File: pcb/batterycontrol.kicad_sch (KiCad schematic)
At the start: 4 parts, among them SW1 MST22D18G2_125

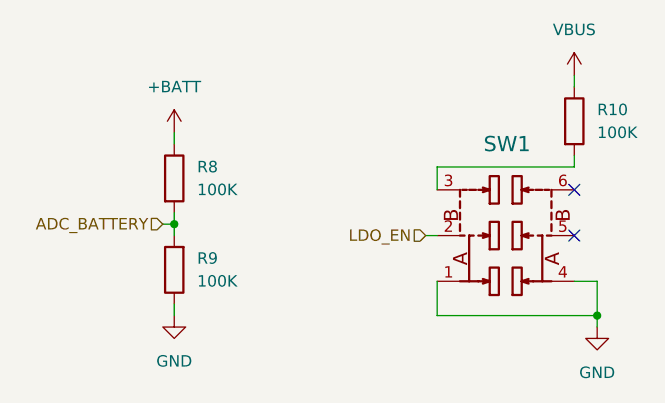
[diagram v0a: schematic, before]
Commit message: schematic done
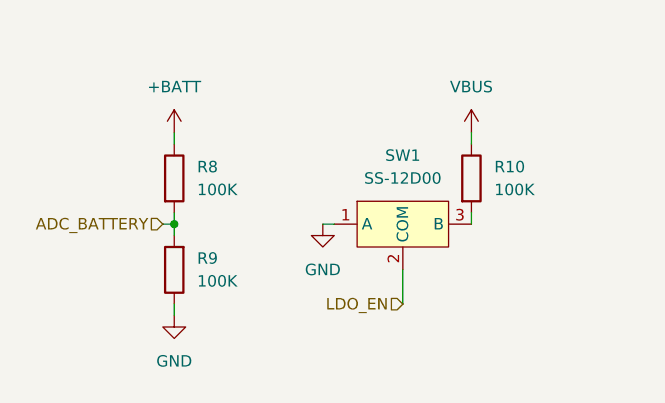
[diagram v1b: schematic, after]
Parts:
- removed SW1: MST22D18G2_125, SlideSwitchSMDTop:SW-SMD_MST22D18G2, symbol MST22D18G2_125:MST22D18G2_125
- added SW1: SS-12D00, SS-12D00:SS12-D00, symbol SS-12D00:SS-12D00
- R10, R8, R9: footprint (none) -> Resistor_SMD:R_0603_1608Metric
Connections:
- net GND: now also SW1.1 (A)
- net LDO_EN: now also SW1.2 (COM)
- net at R10.2: now also SW1.3 (B)
- no-connect marks 2 -> 0
